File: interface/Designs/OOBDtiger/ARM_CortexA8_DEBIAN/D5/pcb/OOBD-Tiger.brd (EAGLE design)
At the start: 63.4 x 38.2 mm, 105 parts, among them IC3 DS3231, U1 SN65HVD230(SO8), U2 SN65HVD230(SO8), U3 SY6280, U4 SY6280, U5 MP1482, U6 TLV70215

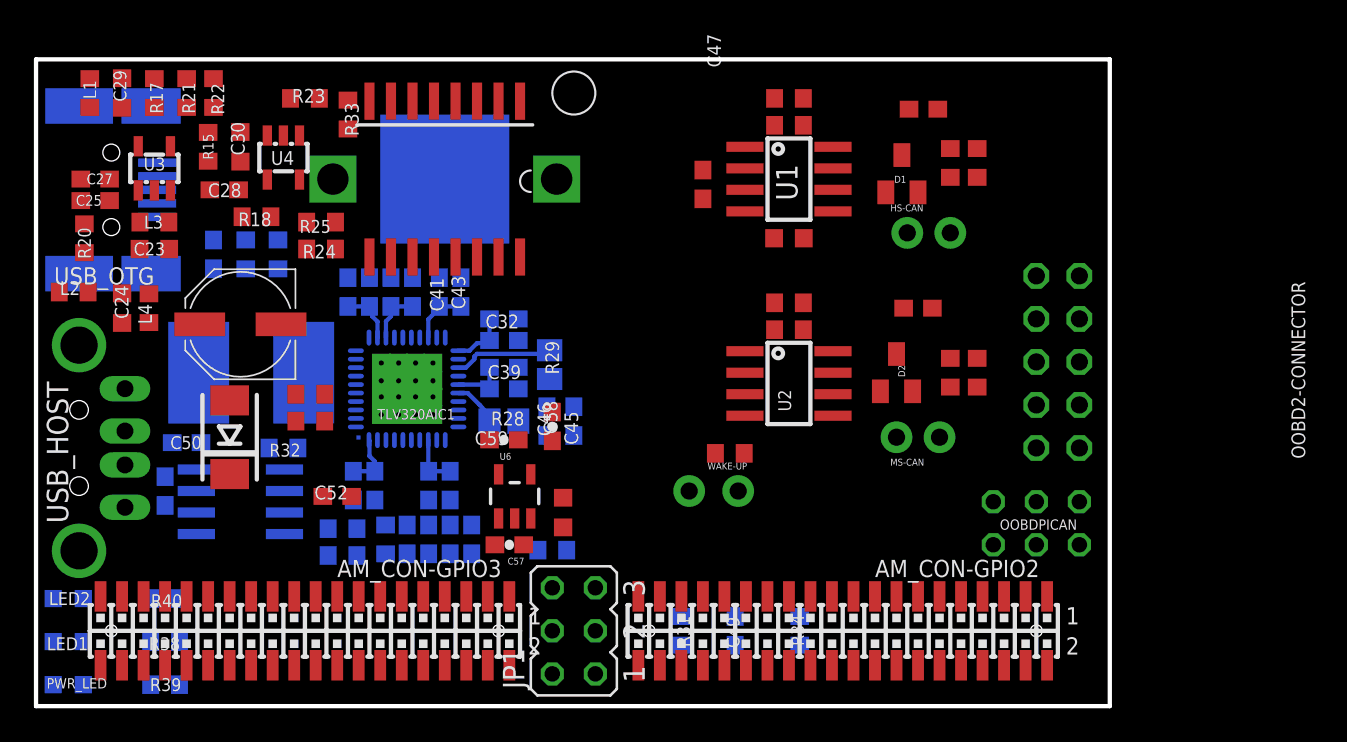
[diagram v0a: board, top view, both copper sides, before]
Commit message: add initial version of OOBDpiZero rearrange Eagle library files
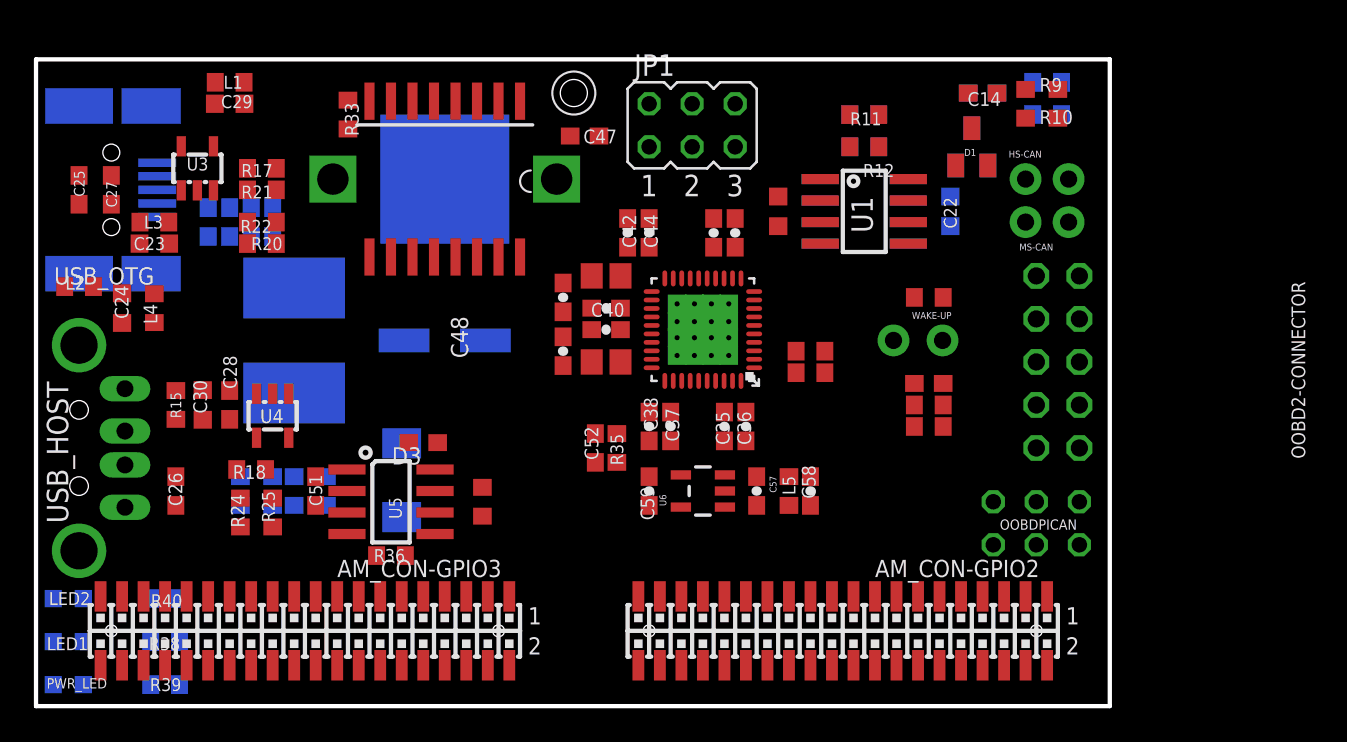
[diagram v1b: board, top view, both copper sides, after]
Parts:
- removed C31, C33: 10µF, SparkFun-Passives:0603-CAP
- removed C32, C34: 0.1µF, SparkFun-Passives:0603-CAP
- moved JP1 30.7 mm to (38.7, 34.3), turned to 0 degrees
- moved R26 29.7 mm to (45.7, 19.7)
- moved R27 29.6 mm to (45.7, 21.0)
- moved C22 29.0 mm to (54.0, 29.2), flipped to the bottom
- moved C56 24.4 mm to (10.2, 28.6)
- moved R23 23.2 mm to (15.2, 12.7), flipped to the bottom, turned to 90 degrees
- moved C55 22.8 mm to (11.4, 28.6)
- moved C35 22.2 mm to (40.6, 16.5), flipped to the top, turned to 270 degrees
- moved C36 22.2 mm to (41.9, 16.5), flipped to the top, turned to 270 degrees
- moved C54 21.5 mm to (12.7, 28.6)
- moved C53 20.3 mm to (14.0, 28.6)
- moved R31 19.8 mm to (52.7, 17.8), flipped to the top, turned to 0 degrees
- moved C49 18.5 mm to (52.7, 19.1), flipped to the top, turned to 0 degrees
- moved C44 18.1 mm to (36.2, 27.9), flipped to the top
- moved R9 18.1 mm to (59.7, 36.8), flipped to the bottom, turned to 0 degrees
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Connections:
- net +3V3: now also AM3352-SOM-EVB-PLATFORM.3-3; no longer C31.2, C32.2, C33.2, C34.2
- net 3V3: no longer AM3352-SOM-EVB-PLATFORM.3-3
- net GND: no longer C31.1, C32.1, C33.1, C34.1
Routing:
- net +3V3: track 16.5 -> 0.00 mm
- net N$18: track 5.91 -> 0.00 mm
- net +5V: track 3.30 -> 0.00 mm
- net DVDD: track 3.12 -> 0.00 mm
- net N$17: track 2.73 -> 0.00 mm
